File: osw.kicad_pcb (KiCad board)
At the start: 4 copper layers, 45 x 41 mm, 67 parts, among them J1 Conn_01x02, Q1 2N7002, SW1 SW_Push, SW2 SW_Push, SW4 SW_Push, SW5 SW_Push, U1 DS3231MZ, U10 XC6209, U11 MCP73831T-2ACI_OT, U12 USBLC6-2SC6, U13 XC6209, U2 BMA400, U3 BMP280, U4 GC9A01_IPS_display, U5 USB-OTG, U6 CH340E, U7 ttgo-32-micro, U8 Quectel_L96, U9 TPS2115A

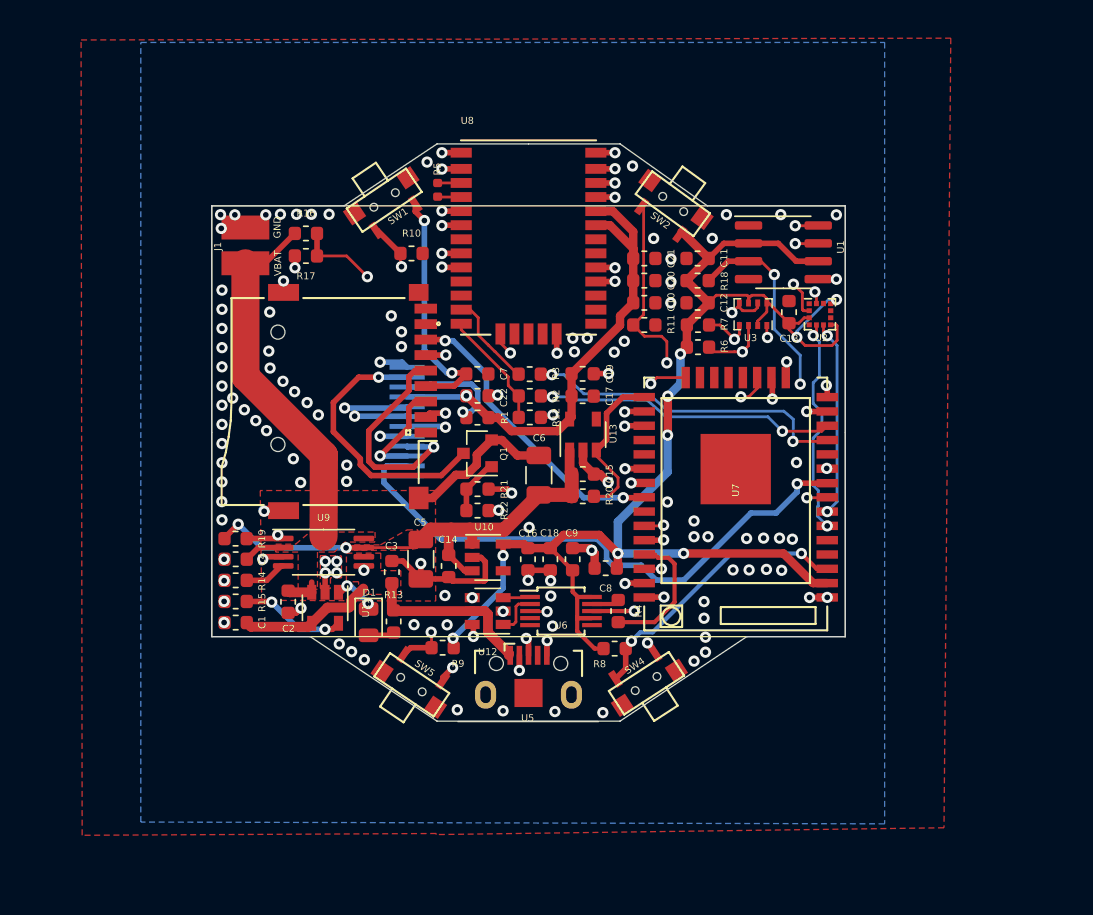
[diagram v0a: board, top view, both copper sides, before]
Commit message: finalize rev 3.0
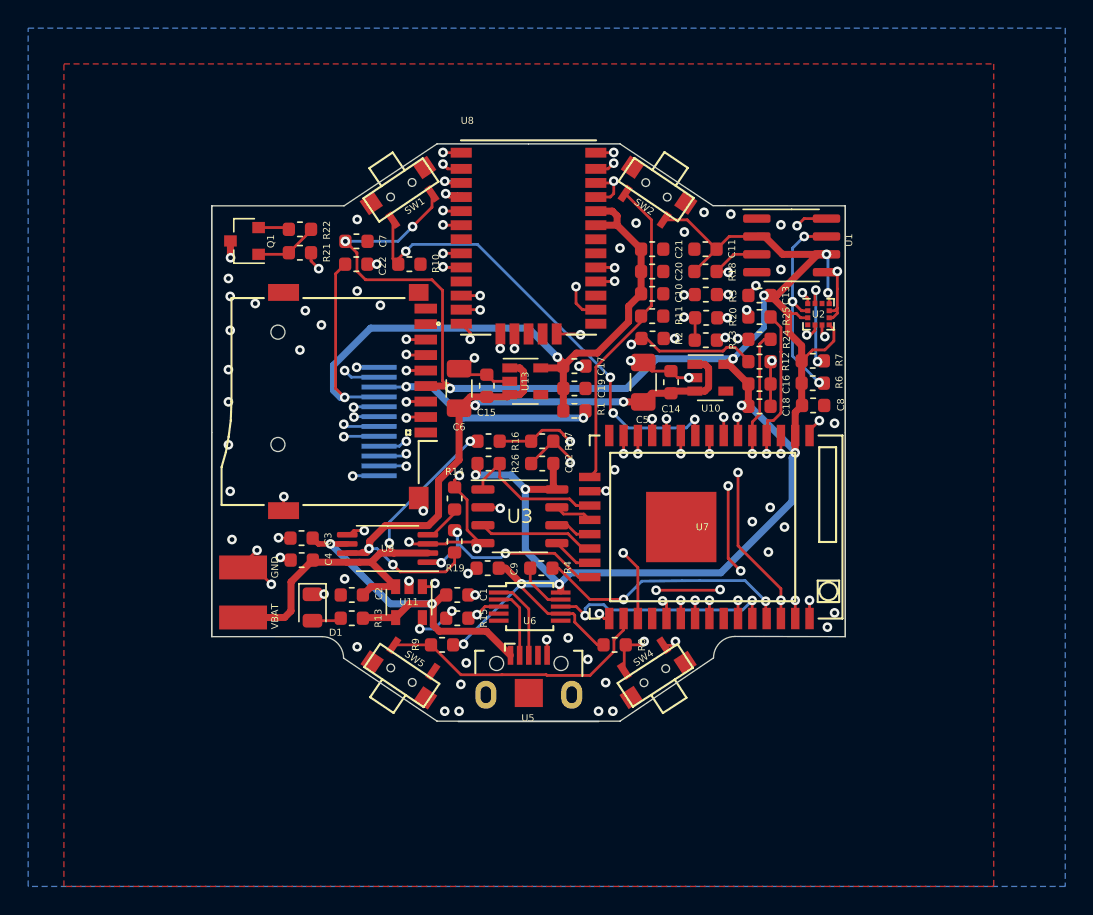
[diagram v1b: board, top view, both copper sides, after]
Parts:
- removed U12: USBLC6-2SC6, Package_TO_SOT_SMD:SOT-23-6
- added G***: LOGO, footprints:aisler_15x12mm, B.Cu at (160.3, 116.3)
- added R23: 56k, Resistor_SMD:R_0603_1608Metric, F.Cu at (172.6, 103.4)
- added R24: 1k, Resistor_SMD:R_0603_1608Metric, F.Cu at (176.4, 103.4)
- added R25: 1k, Resistor_SMD:R_0603_1608Metric, F.Cu at (176.4, 101.8)
- added R26: 10k, Resistor_SMD:R_0603_1608Metric, F.Cu at (157.2, 112.2)
- R16: value 1M -> 200k
- R17: value 220k -> 10k
- R19: value 2.2K -> 200k
- R20: value 2.2K -> 10k
- R5: moved to B.Cu
- U3: value BMP280 -> PSRAM64H; footprint open-Smartwatch:Bosch_LGA-8_2x2.5mm_P0.65mm_ClockwisePinNumbering -> Package_SO:SOP-8_3.9x4.9mm_P1.27mm
- moved J1 24.7 mm to (139.7, 122.6)
- moved R22 23.6 mm to (143.8, 95.6), turned to 0 degrees
- moved Q1 22.4 mm to (139.8, 96.4)
- moved U3 21.9 mm to (159.4, 116.0), turned to 0 degrees
- moved R17 21.3 mm to (161.0, 110.6), turned to 0 degrees
- moved R21 21.0 mm to (143.8, 97.2)
- moved C16 20.6 mm to (176.4, 106.6), turned to 0 degrees
- moved C14 20.5 mm to (170.1, 106.4), turned to 90 degrees
- moved U10 20.3 mm to (172.9, 106.1)
- moved C5 20.2 mm to (168.1, 106.4), turned to 90 degrees
- moved R16 19.6 mm to (157.2, 110.6)
- moved C8 18.7 mm to (180.2, 108.1), turned to 0 degrees
- moved C18 18.4 mm to (176.4, 108.1), turned to 0 degrees
- moved R12 16.8 mm to (176.4, 105.0)
- moved R14 16.6 mm to (154.7, 114.7), turned to 90 degrees
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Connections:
- R20 pad 1: /VCC -> /GPS_FON2V8
- R20 pad 2: /PWR2_EN -> /GPS_FON3V3
- U13 pad 3: /PWR2_EN -> /VCC
- U2 pad 1: Net-(U2-Pad1) -> GND
- U3 pad 1: GND -> /GPIO10
- U3 pad 2: +3V3 -> /SD0
- U3 pad 3: /SDA -> /SD3
- U3 pad 4: /SCL -> GND
- U3 pad 5: GND -> /SD1
- U3 pad 6: +3V3 -> /CLK
- U3 pad 7: GND -> /SD2
- U5 pad 3: /D2_P -> /D_P
- U5 pad 4: /D2_N -> /D_N
- U6 pad 1: /D1_P -> /D_P
- U6 pad 2: /D1_N -> /D_N
- U7 pad 11: Net-(U7-Pad11) -> /GPS_FON3V3
- U7 pad 18: /BTN2 -> /GPIO10
- U7 pad 19: Net-(U7-Pad19) -> /SD2
- U7 pad 20: Net-(U7-Pad20) -> /CLK
- U7 pad 21: Net-(U7-Pad21) -> /SD3
- U7 pad 22: Net-(U7-Pad22) -> /SD1
- U7 pad 24: /PWR2_EN -> /TFT_RST
- U7 pad 28: Net-(U7-Pad28) -> /SD0
- U7 pad 4: Net-(U7-Pad4) -> /3DFIX_3V3
- U7 pad 5: Net-(U7-Pad5) -> /GEO_F3V3
- U7 pad 9: /TFT_RST -> /BTN2
- U8 pad 2: Net-(U8-Pad2) -> /3DFIX_2V8
- U8 pad 24: Net-(U8-Pad24) -> /GEO_F2V8
- U8 pad 28: Net-(U8-Pad28) -> /GPS_FON2V8
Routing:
- net /B_MON: track 47.8 -> 15.2 mm
- net +3V3: track 138.0 -> 164.9 mm, vias 11 -> 14
- net /STAT_PWR: track 40.1 -> 15.2 mm, vias 2 -> 3
- net /GEO_F2V8: track 0.00 -> 24.3 mm, vias 0 -> 2
- net /3V3_2: track 35.6 -> 56.4 mm, vias 1 -> 2
- net /TFT_RST: track 40.7 -> 21.1 mm, vias 1 -> 2
- net /3DFIX_2V8: track 0.00 -> 19.1 mm, vias 0 -> 2
- net /FLASH: track 37.3 -> 19.9 mm, vias 2 -> 0
- net /SD0: track 0.00 -> 17.0 mm, vias 0 -> 2
- net /VCC: track 35.8 -> 52.6 mm, vias 2 -> 4
- net /GPS_FON2V8: track 0.00 -> 16.4 mm, vias 0 -> 2
- net /GPS_RX2V8: track 8.34 -> 23.2 mm, vias 0 -> 2
- net /MISO: track 21.3 -> 32.8 mm
- net /PWR2_EN: track 11.4 -> 0.00 mm
- net /TFT_CS: track 21.7 -> 32.8 mm
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- added copper zone on In1.Cu, net GND
- added copper zone on In2.Cu, net GND
- removed copper zone on F.Cu, net /VBAT
- removed copper zone on F.Cu, net /VBUS
- removed copper zone on F.Cu, net /VCC
- removed copper zone on GND, net GND
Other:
- outline, holes or cut-outs redrawn
- board text added: "1"
- board text added: "2"
- board text added: "3"
- board text added: "@pauls_3d_things"
- board text added: "R"
- board text added: "V 3.0"
- board text removed: "BTN1"
- board text removed: "BTN2"
- board text removed: "BTN3"
- board text removed: "RESET"
- board text removed: "V 2.1"
- board text removed: "pauls_3d_things"
